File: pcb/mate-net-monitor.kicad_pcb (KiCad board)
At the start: 2 copper layers, 65 parts, among them J1 RJHSE-5081, J2 Conn_02x04_Odd_Even, J3 Conn_02x02_Odd_Even, J4 6P6C, J5 6P6C, Q1 Si2337DS, U1 LM5085MY, U2 TLP185, U3 TLP185, U4 TLP185, U5 MAX3485

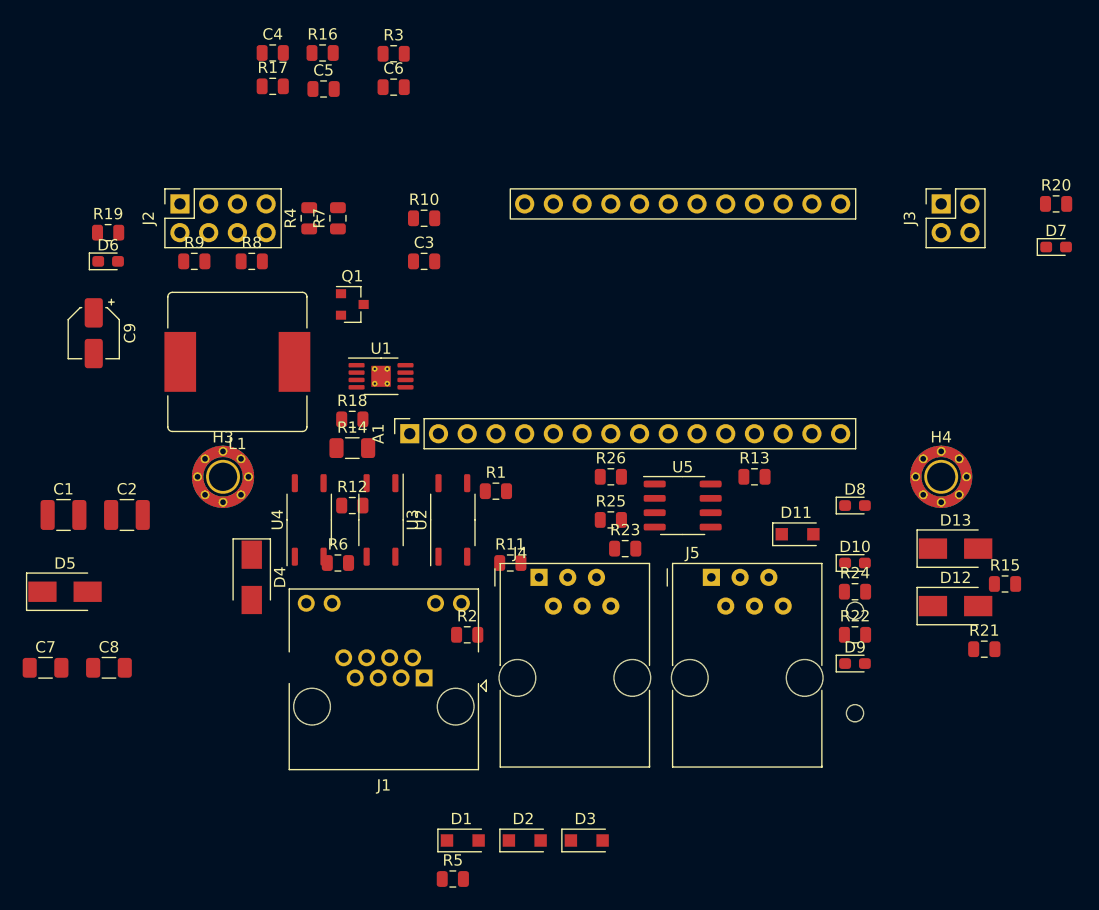
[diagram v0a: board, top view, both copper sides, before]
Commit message: layout P1
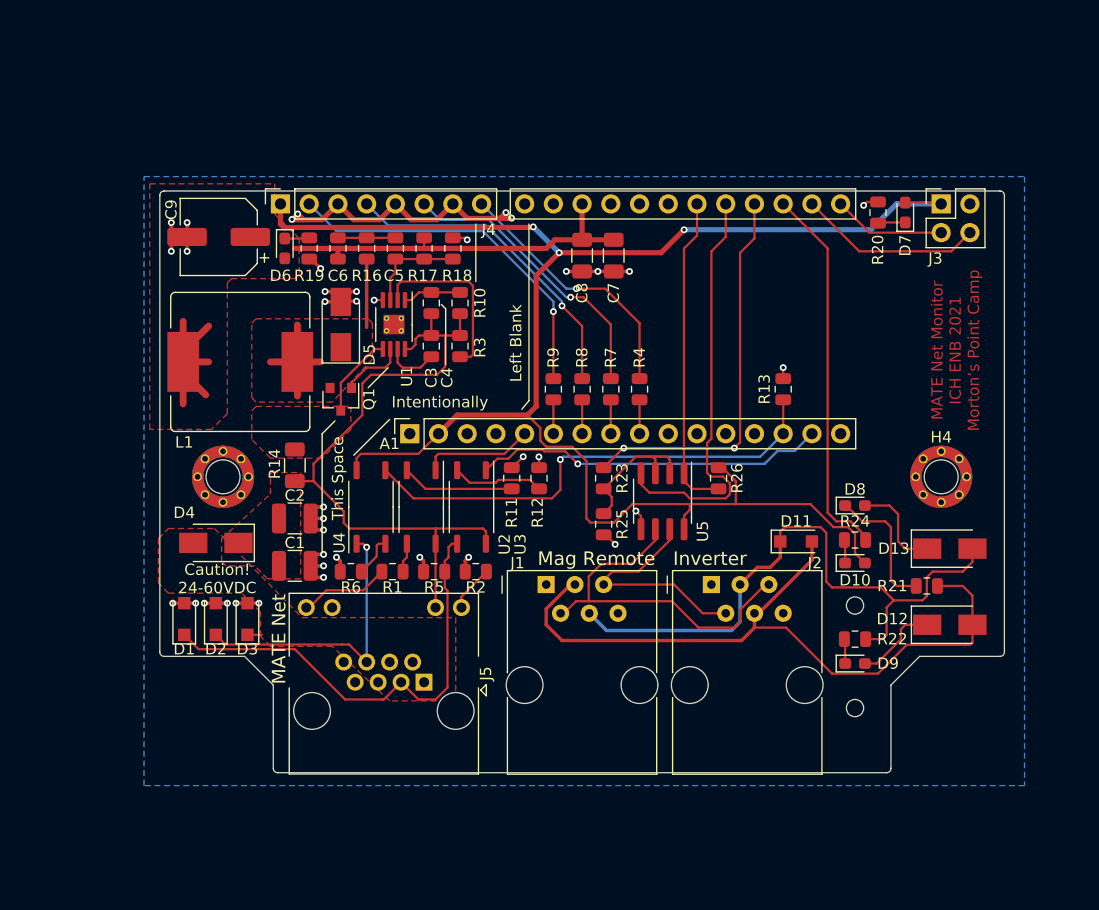
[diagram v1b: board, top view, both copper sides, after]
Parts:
- removed the J2 at (114.3, 72.4)
- removed R15: 0, Resistor_SMD:R_0805_2012Metric
- added J4: Conn_01x08, Connector_PinSocket_2.54mm:PinSocket_1x08_P2.54mm_Vertical, F.Cu at (123.2, 72.4)
- C9: value ?uF -> 180uF; footprint Capacitor_SMD:CP_Elec_4x4.5 -> Capacitor_SMD:CP_Elec_6.3x5.9
- R4, R7, R8, R9: value 22 -> 47k
- moved C7 62.1 mm to (152.7, 77.0), turned to 270 degrees
- moved C8 55.5 mm to (149.9, 77.0), turned to 270 degrees
- moved D3 35.8 mm to (120.3, 109.1), turned to 90 degrees
- moved D5 33.9 mm to (128.5, 83.1), turned to 90 degrees
- moved R9 33.7 mm to (147.3, 88.8), turned to 270 degrees
- moved D2 33.6 mm to (117.5, 109.1), turned to 90 degrees
- moved R4 32.9 mm to (154.9, 88.8), turned to 270 degrees
- moved D1 31.5 mm to (114.7, 109.1), turned to 90 degrees
- moved R8 31.3 mm to (149.9, 88.8), turned to 270 degrees
- moved R7 28.5 mm to (152.4, 88.8), turned to 270 degrees
- moved R5 27.2 mm to (136.8, 104.9), turned to 180 degrees
- moved R3 26.5 mm to (139.1, 85.0), turned to 270 degrees
- moved C4 26.2 mm to (136.5, 81.2), turned to 90 degrees
- moved C1 20.9 mm to (124.5, 104.4)
- moved R17 19.6 mm to (135.9, 76.3), turned to 270 degrees
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- renumbered J4 to J1, J5 to J2, J1 to J5
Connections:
- net Net-(C3-Pad2) renamed /P5V_VCC
- net Net-(C4-Pad2) renamed /P5V_ADJ
- net Net-(C5-Pad1) renamed /P5V_AC
- net Net-(D5-Pad1) renamed /P5V_SW
- net Net-(Q1-Pad1) renamed /P5V_PGATE
- net Net-(R23-Pad2) renamed /U5_EN
- A1 pad RST: (no net) -> Net-(A1-PadRST)
- A1 pad VUSB: Net-(A1-PadVUSB) -> +5V
- H3 pad 1: GND -> Net-(H3-Pad1)
- H4 pad 1: GND -> Net-(H4-Pad1)
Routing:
- net +3V3: track 0.00 -> 147.2 mm, vias 0 -> 3
- net GND: track 0.00 -> 69.6 mm, vias 0 -> 39
- net /MAG_NET_GND: track 0.00 -> 63.9 mm
- net +BATT: track 0.00 -> 58.3 mm
- net /MAG_NET_P14V: track 0.00 -> 55.7 mm
- net +5V: track 0.00 -> 51.0 mm
- net /PB_UART1_RX: track 0.00 -> 43.2 mm, vias 0 -> 1
- net /MATE_NET_TXD: track 0.00 -> 40.9 mm
- net /PB_UART2_TX: track 0.00 -> 37.3 mm
- net /PB_D3: track 0.00 -> 34.6 mm, vias 0 -> 2
- net /PB_D2: track 0.00 -> 33.5 mm
- net /MAG_NET_A: track 0.00 -> 32.4 mm
- net /CONN_ADC1: track 0.00 -> 32.0 mm, vias 0 -> 1
- net /PB_UART1_TX: track 0.00 -> 31.2 mm, vias 0 -> 1
- net /CONN_ADC2: track 0.00 -> 28.4 mm, vias 0 -> 1
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- added copper zone on F.Cu, net +5V
- added copper zone on F.Cu, net +BATT
- added copper zone on F.Cu, net /P5V_ISEN
- added copper zone on F.Cu, net /P5V_SW
- added copper zone on F.Cu, net /PBATT_CONN
- added copper zone on B.Cu, net GND
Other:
- board outline added: 74.7 x 51.4 mm
- net class 6/6 added: clearance 0.1524, trace_width 0.1524, via_dia 0.6096, via_drill 0.3048
- net class 8/6 added: clearance 0.1524, trace_width 0.2032, via_dia 0.6096, via_drill 0.3048
- net class Default: clearance 0.2 -> 0.2032; trace_width 0.25 -> 0.2032; via_dia 0.8 -> 0.6096; via_drill 0.4 -> 0.3048
- rule trace_clearance: 0.2 -> 0.2032
- rule trace_min: 0.2 -> 0.1524
- rule via_min_size: 0.4 -> 0.3048
- board text added: "Caution! 24-60VDC"
- board text added: "Intentionally"
- board text added: "Inverter"
- board text added: "Left Blank"
- board text added: "MATE Net"
- board text added: "MATE Net Monitor ICH ENB 2021 Morton’s Point Camp"
- board text added: "Mag Remote"
- board text added: "This Space"
